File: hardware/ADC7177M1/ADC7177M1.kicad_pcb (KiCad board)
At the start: 6 copper layers, 54 x 29 mm, 133 parts, among them J1 3670513, J2 3670345, J3 FTSH-108-04-L-DV, J4 FTSH-108-04-L-DV, U1 ADG1419BRMZ, U10 ADP7182ACPZN, U11 ADA4522-2ARMZ, U12 AD8066ARMZ, U13 AD7177-2BRUZ, U14 ADR1399KEZ, U15 LT1012S8, U16 ADA4522-1ARMZ, U17 AD8065ART, U2 ADG1419BRMZ, U3 OPA2189IDGK, U4 OPA2388IDGKx, U5 AD8066ARMZ, U6 ADG1408YRUZ, U7 ADG1408YRUZ, U8 ADP7118ACPZN, U9 ADP7118ACPZN, Y1 ECS-2520MV-160-BL-TR

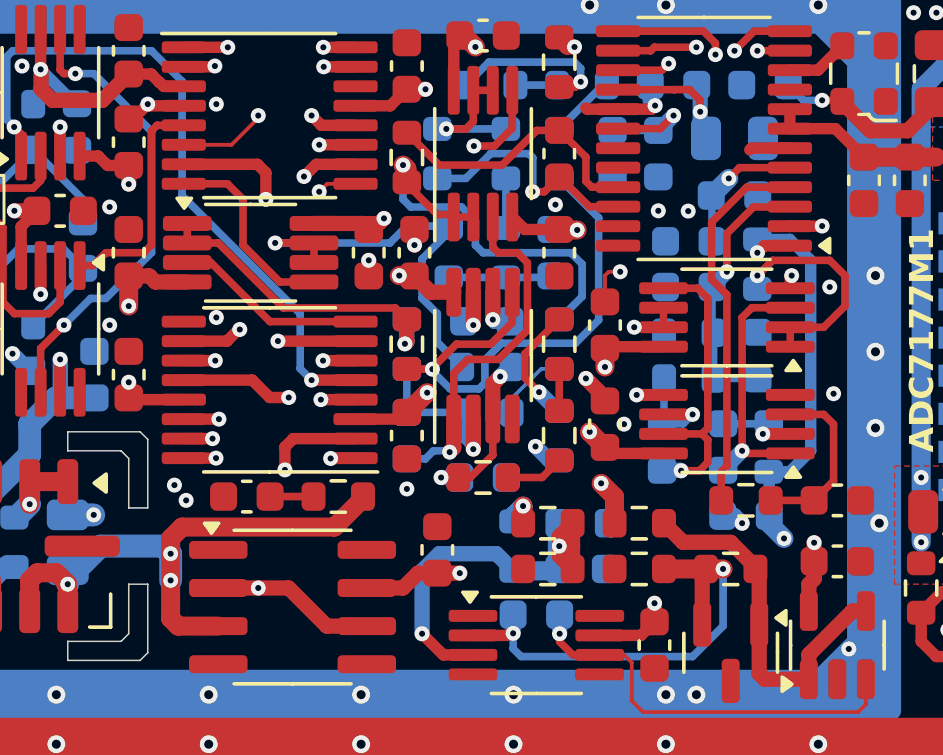
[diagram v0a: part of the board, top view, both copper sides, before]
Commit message: PCB
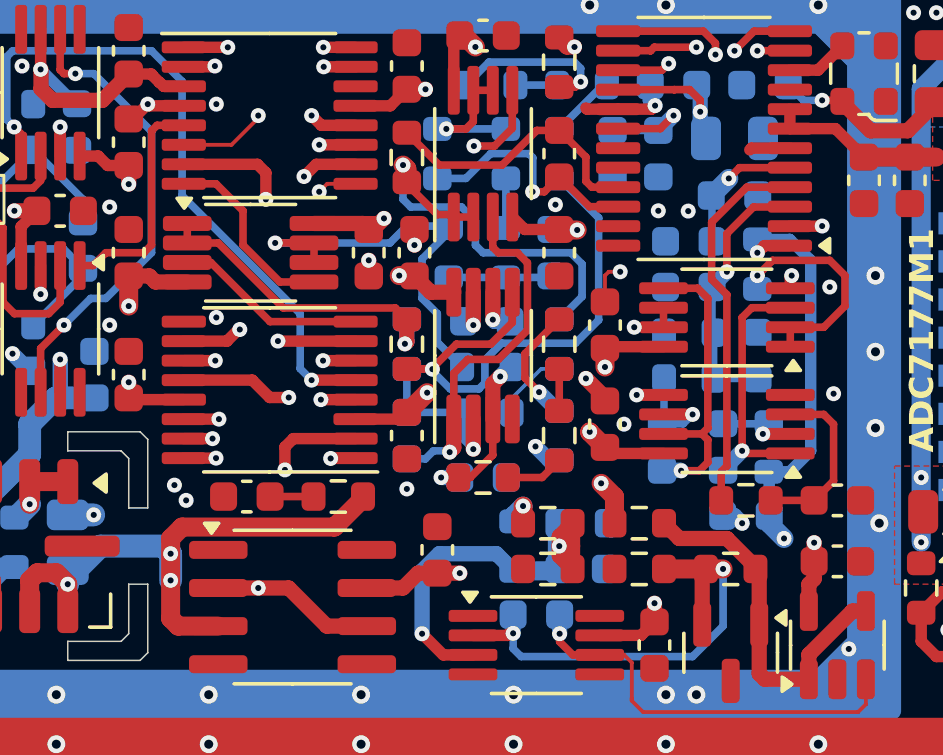
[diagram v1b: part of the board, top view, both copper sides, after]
